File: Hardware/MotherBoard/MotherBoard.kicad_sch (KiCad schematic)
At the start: 16 parts, among them J1 POWER, J10 I/O_PWR, J2 I/O0, J5 I/O1, J6 EXTRN_CLCK, U1 AMS1117-5.0

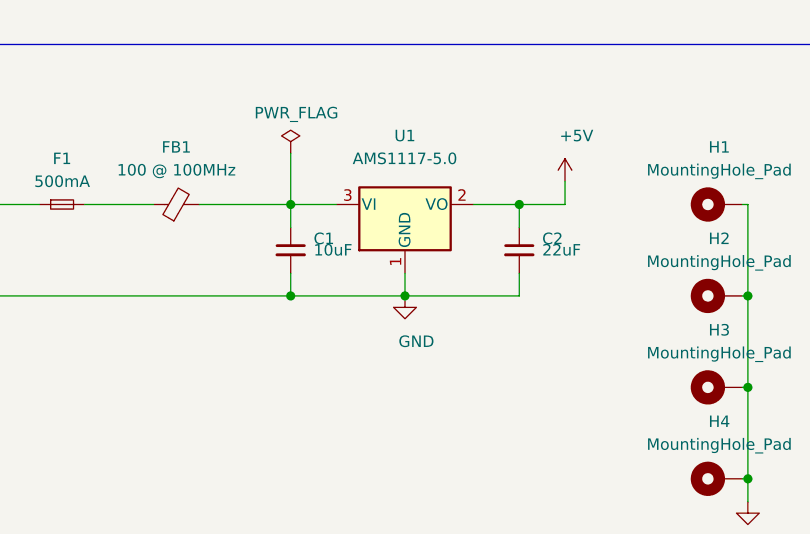
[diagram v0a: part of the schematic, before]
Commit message: Finalize daughter board
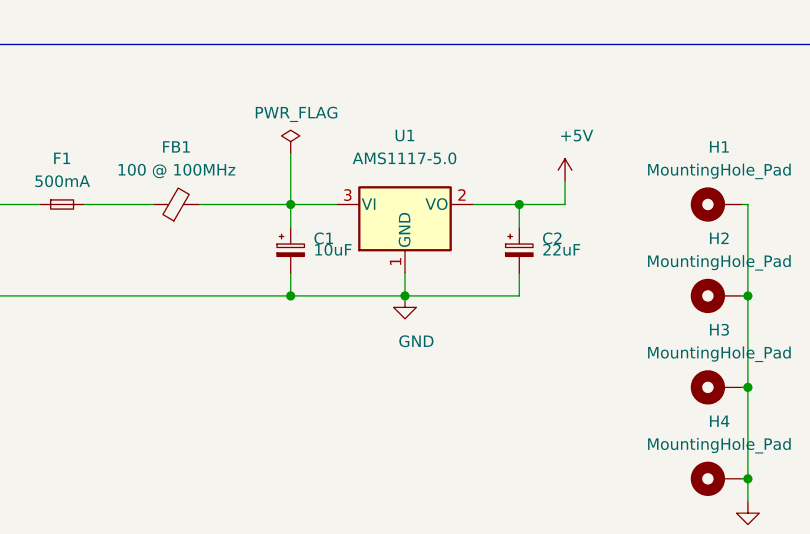
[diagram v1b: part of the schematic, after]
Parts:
- C1, C2: symbol Device:C_Small -> Device:CP_Small
- U1: footprint Package_TO_SOT_SMD:SOT-223-3_TabPin2 -> Package_TO_SOT_THT:TO-220-3_Horizontal_TabDown
